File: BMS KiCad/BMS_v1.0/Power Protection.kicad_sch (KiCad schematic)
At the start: 8 parts, among them J1 Conn_01x02, J2 Conn_01x02, Q1 PMOS, Q2 PMOS, U2 INA193

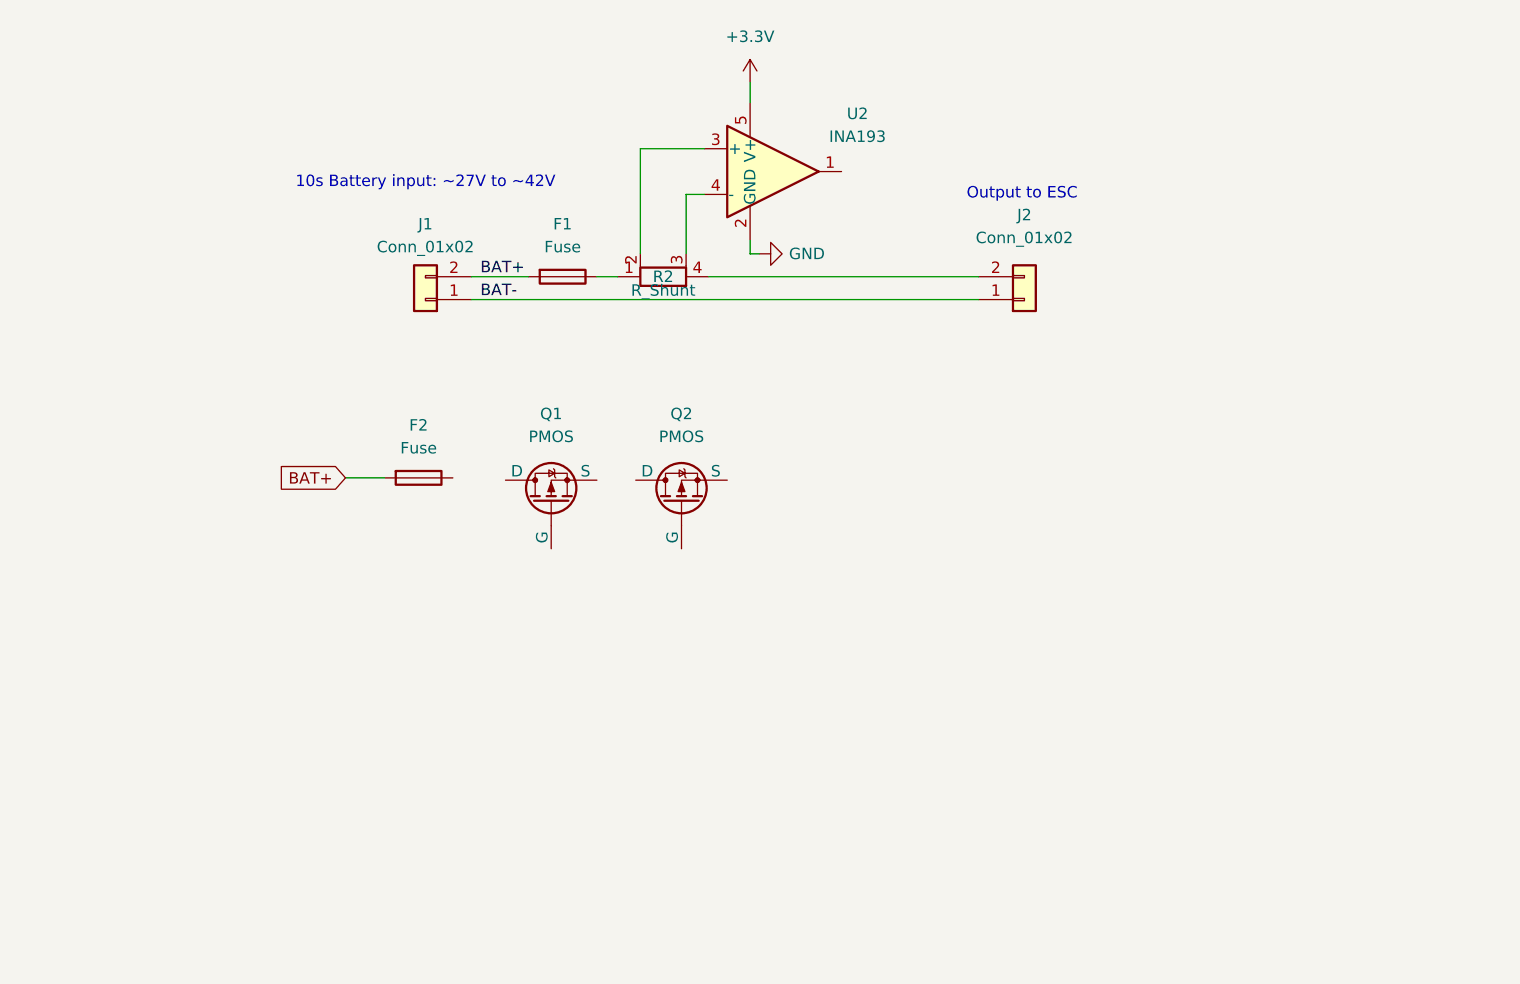
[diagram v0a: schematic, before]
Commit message: power protection done pretty much
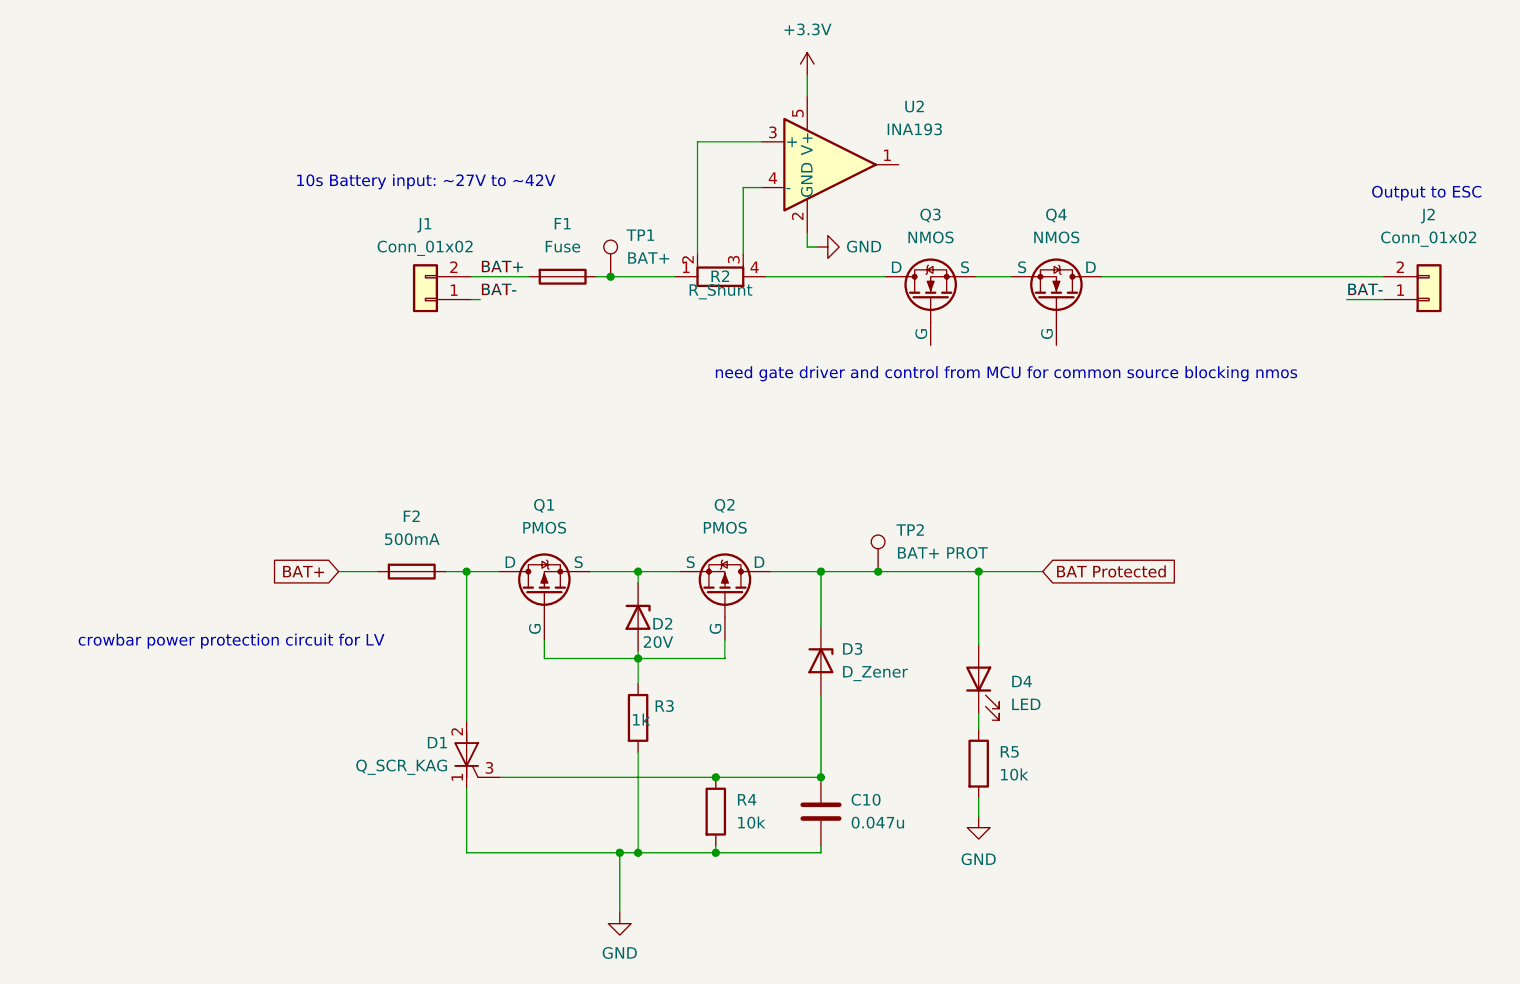
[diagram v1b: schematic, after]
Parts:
- added C10: 0.047u, symbol Device:C
- added D1: Q_SCR_KAG, symbol Device:Q_SCR_KAG
- added D2: 20V, symbol Device:D_Zener
- added D3: D_Zener, symbol Device:D_Zener
- added D4: LED, symbol Device:LED
- added Q3, Q4: NMOS, symbol Simulation_SPICE:NMOS
- added R3: 1k, symbol Device:R
- added R4, R5: 10k, symbol Device:R
- added TP1: BAT+, symbol Connector:TestPoint
- added TP2: BAT+ PROT, symbol Connector:TestPoint
- F2: value Fuse -> 500mA
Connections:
- net GND: now also C10.2, D1.1 (K), R3.2, R4.2, R5.2
- net at F2.1: now also Q1.1 (D), D1.2 (A)
- net at F1.1, R2.1: now also TP1.1
- net at R2.4: now also Q3.1 (D); no longer J2.2 (Pin_2)
- net at Q1.2 (G): now also Q2.2 (G), D2.2 (A), R3.1
- net at Q1.3 (S): now also Q2.3 (S), D2.1 (K)
- net BAT Protected: now reaches Q2.1 (D)
- net BAT Protected: now also D3.1 (K), D4.2 (A), TP2.1
- new net: C10.1, D1.3 (G), D3.2 (A), R4.1
- new net: Q3.3 (S), Q4.3 (S)
- new net: D4.1 (K), R5.1
- new net: J2.2 (Pin_2), Q4.1 (D)
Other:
- note added: "crowbar power protection circuit for LV"
- note added: "need gate driver and control from MCU for common source blocking nmos"
- moved on the sheet: F2, J2, Q1, Q2, R2, U2
